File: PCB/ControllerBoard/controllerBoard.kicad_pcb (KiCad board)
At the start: 2 copper layers, 129 x 83.8 mm, 60 parts, among them J1 Conn_02x06_Odd_Even, J2 Conn_02x06_Odd_Even, SW1 SW_Push, SW2 SW_Push, SW3 SW_Push, SW4 SW_Push, SW5 SW_Push, SW6 SW_Push, SW7 SW_Push, SW8 SW_Push, U1 MCP3008

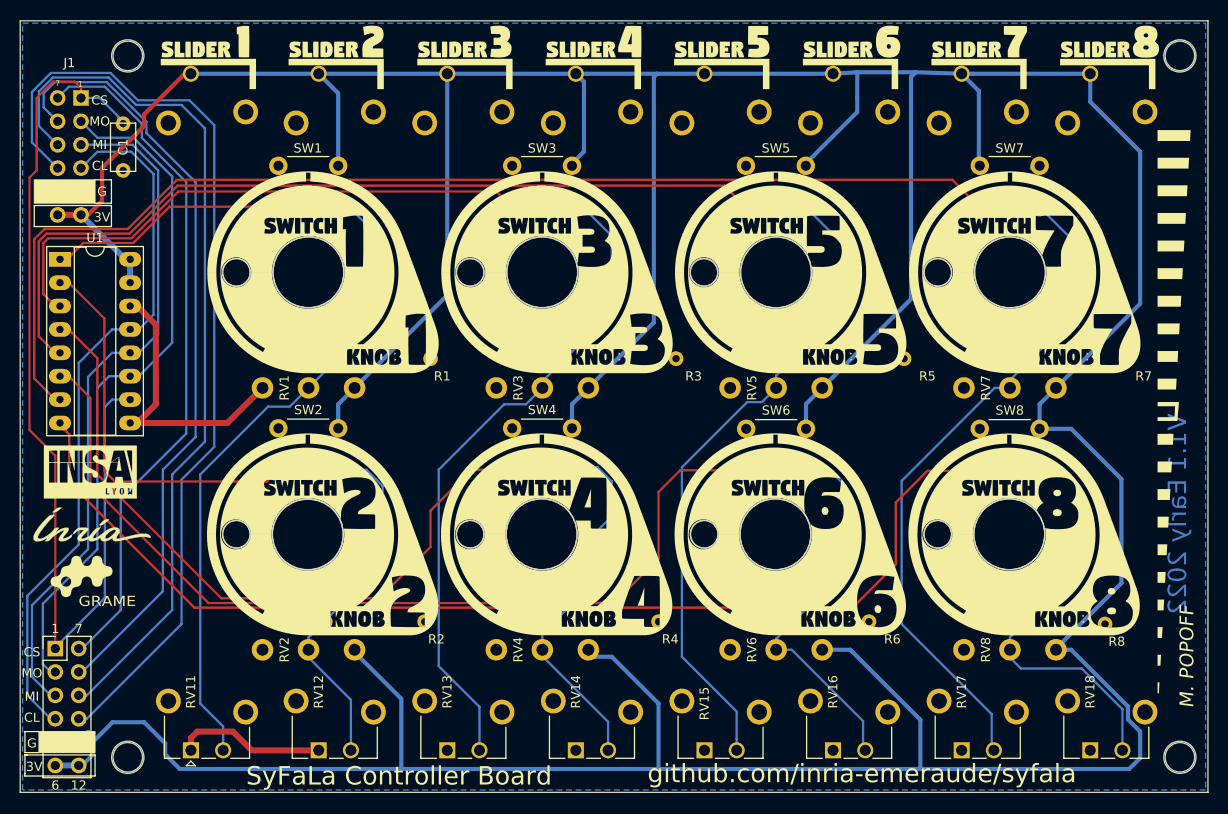
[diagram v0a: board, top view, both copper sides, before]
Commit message: [general] main update
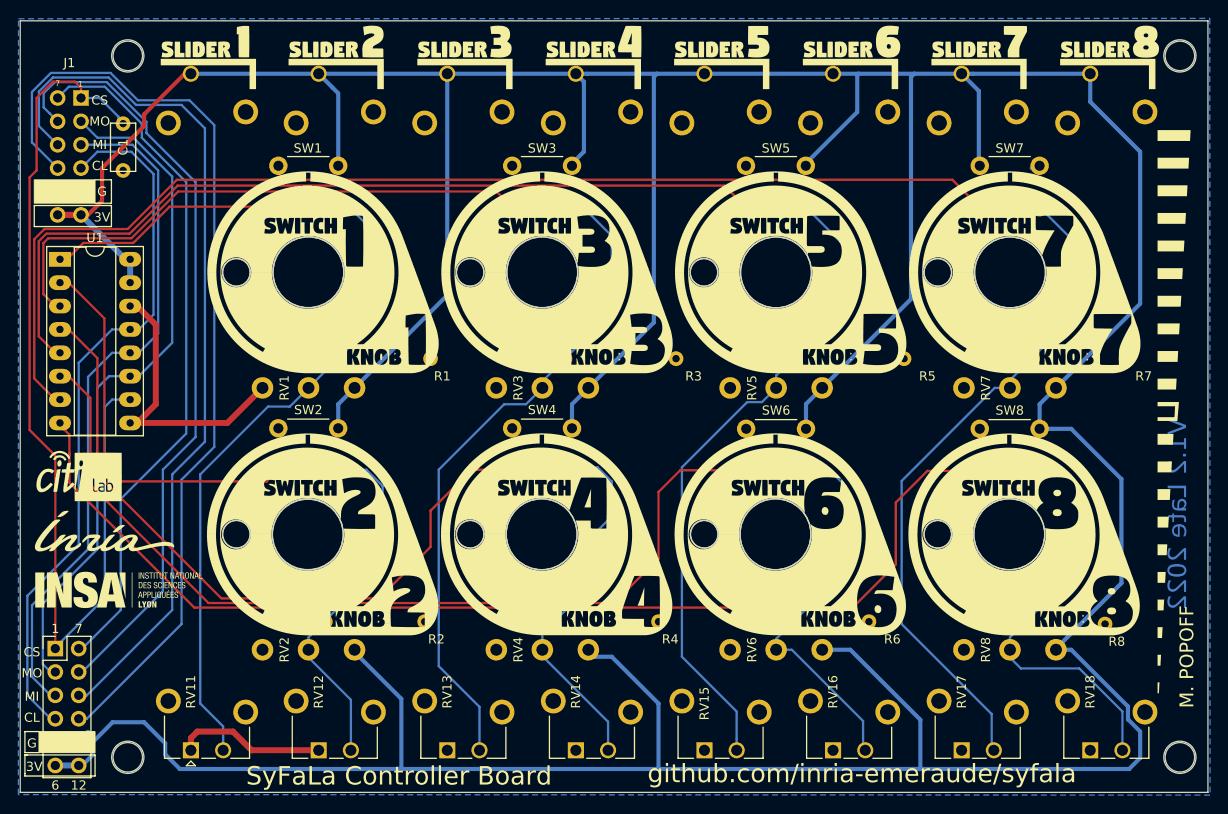
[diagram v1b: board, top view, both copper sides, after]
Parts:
- removed the svg2mod at (49.1, 77.7)
- removed the svg2mod at (50.2, 72.0)
- removed the svg2mod at (50.0, 66.3)
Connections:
- RV8 pad 3: Net-(RV8-Pad3) -> GND
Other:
- net class Default removed
- net class VCC removed
- board text added: "V1.2 Late 2022"
- board text removed: "GRAME"
- board text removed: "V1.1 Early 2022"

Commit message: [linux] dev/linux branch
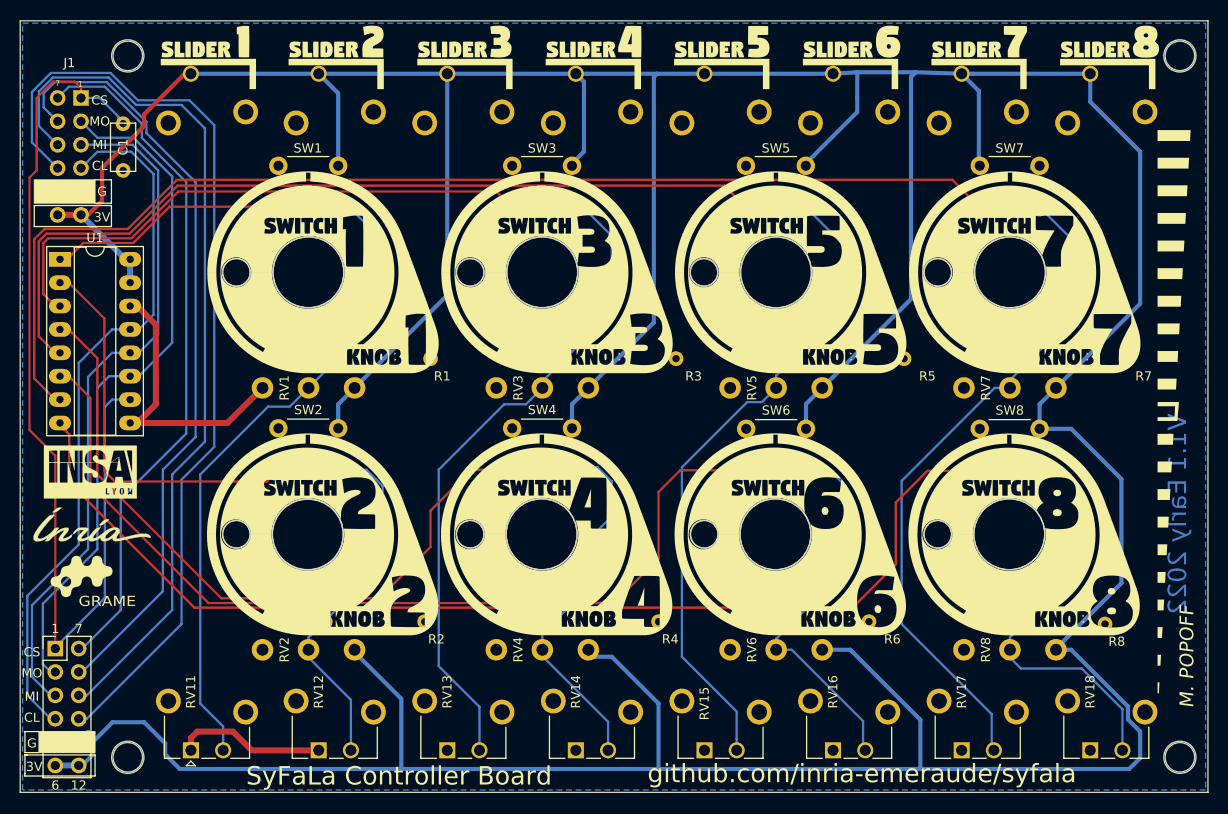
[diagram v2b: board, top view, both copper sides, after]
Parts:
- added svg2mod: G***, grame, F.Cu at (49.1, 77.7)
- added svg2mod: G***, inria, F.Cu at (50.2, 72.0)
- added svg2mod: G***, INSA, F.Cu at (50.0, 66.3)
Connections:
- RV8 pad 3: GND -> Net-(RV8-Pad3)
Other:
- net class Default added: clearance 0.25, trace_width 0.25, via_dia 0.8, via_drill 0.4
- net class VCC added: clearance 0.25, trace_width 0.35, via_dia 0.8, via_drill 0.4
- board text added: "GRAME"
- board text added: "V1.1 Early 2022"
- board text removed: "V1.2 Late 2022"
